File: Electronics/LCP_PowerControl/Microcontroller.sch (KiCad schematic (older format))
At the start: 22 parts, among them J5 Conn_02x05_Odd_Even, J6 Conn_02x06_Odd_Even, J7 Conn_02x02_Odd_Even, J8 Conn_02x02_Odd_Even, SW1 SW_Push, U3 MSP430FR5989, Y1 32.768kHz

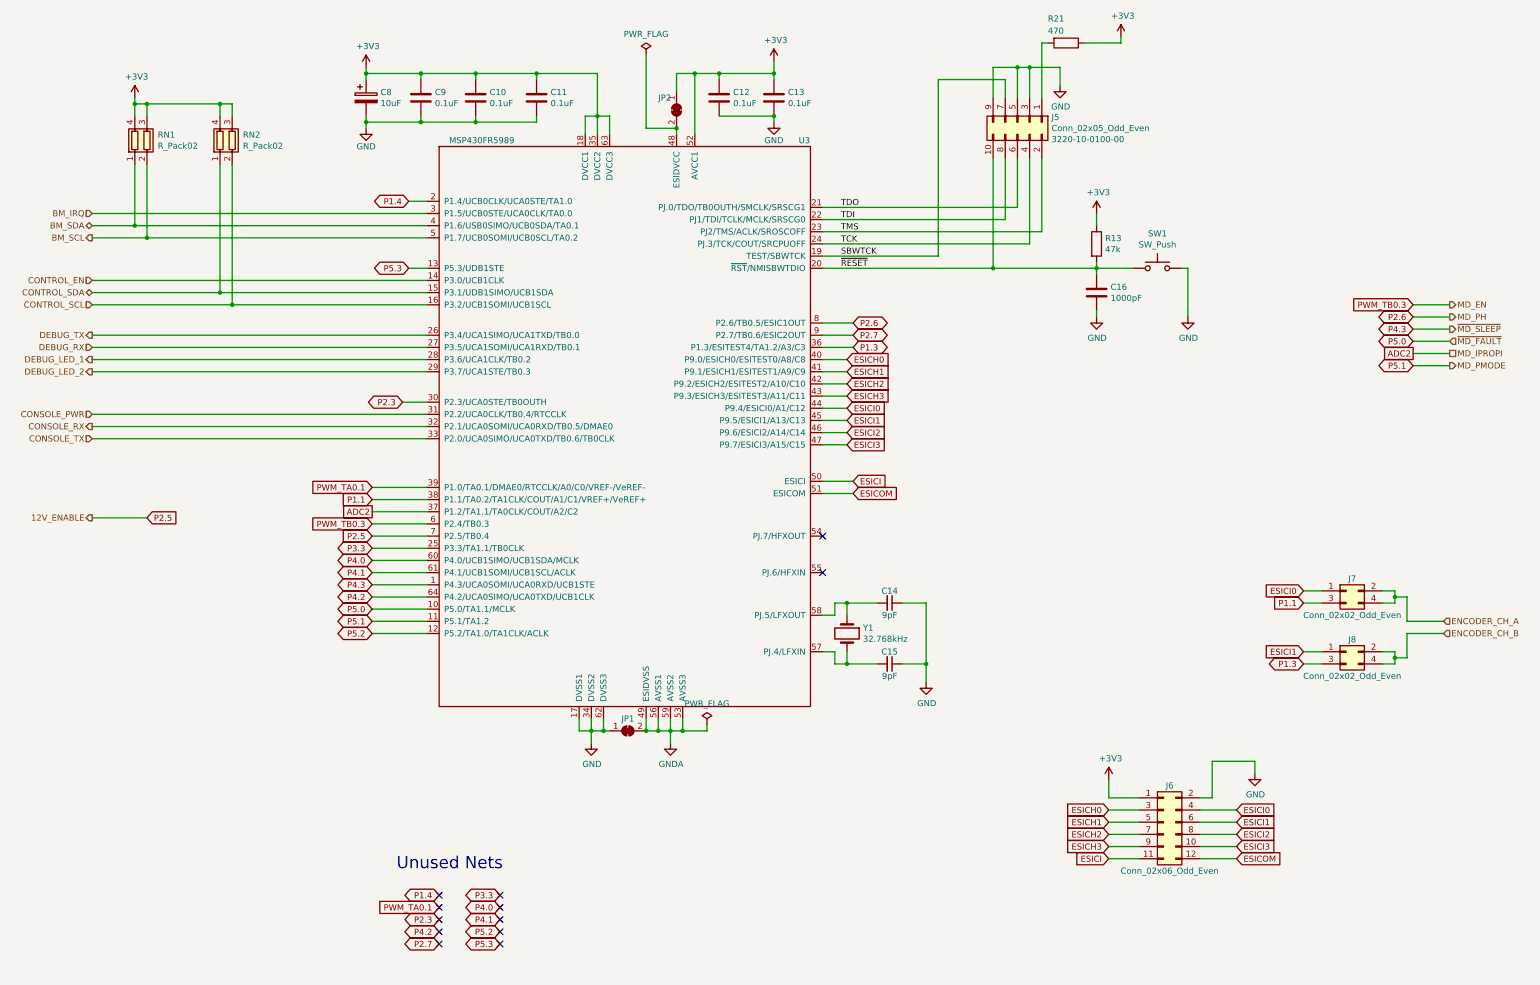
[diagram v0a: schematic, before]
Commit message: Rev 1 Update
Issues #9-#13 fixed
Rev 1 Gerbers & BOM Ready
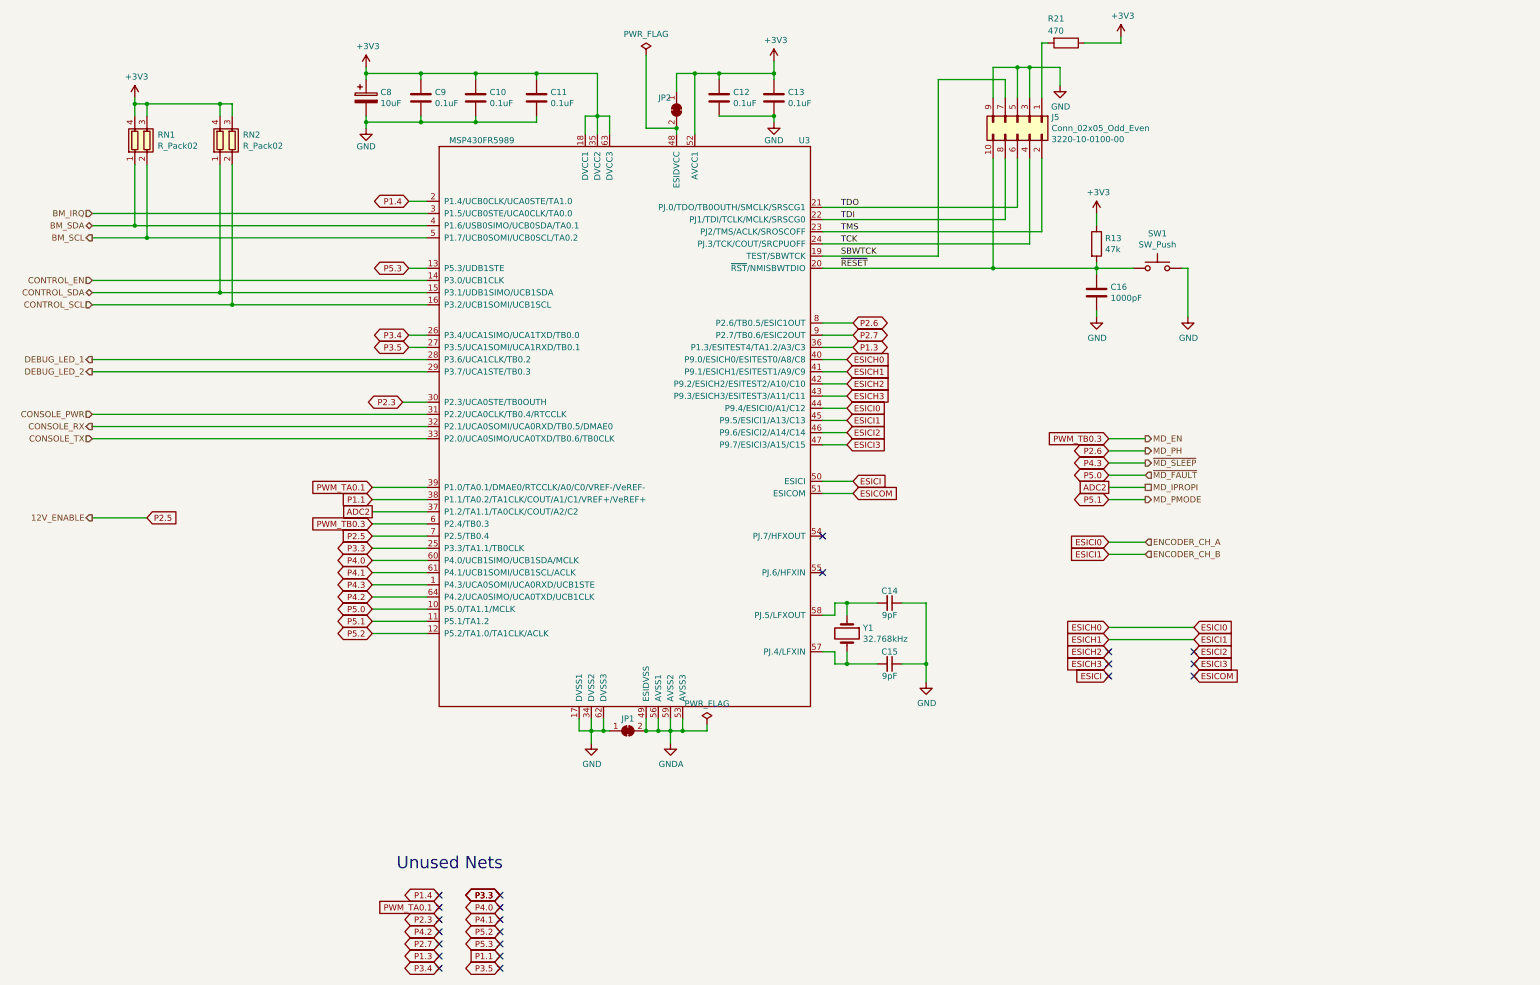
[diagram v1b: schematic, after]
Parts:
- removed J6: Conn_02x06_Odd_Even, Connector_PinHeader_2.00mm:PinHeader_2x06_P2.00mm_Vertical, symbol Connector_Generic:Conn_02x06_Odd_Even
- removed J7, J8: Conn_02x02_Odd_Even, Connector_PinHeader_2.00mm:PinHeader_2x02_P2.00mm_Vertical, symbol Connector_Generic:Conn_02x02_Odd_Even
- C14, C15: MPN CBR06C909B5GAC -> CBR06C909BAGAC
- C16: MPN GCJ188R72A102KA01D -> CL10B102KB8NNNC
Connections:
- net ESICI0 is gone; now on net ESICH0: U3.44 (P9.4/ESICI0/A1/C12)
- net ESICI1 is gone; now on net ESICH1: U3.45 (P9.5/ESICI1/A13/C13)
- net DEBUG_RX renamed P3.5
- net DEBUG_TX renamed P3.4
- no-connect marks 12 -> 22
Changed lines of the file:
@@
 Text HLabel 3900 4800 0    50   Output ~ 0
 CONSOLE_RX
-Text HLabel 15050 3800 2    50   Output ~ 0
+Text HLabel 12550 4900 2    50   Output ~ 0
 MD_EN
-Text HLabel 15050 3900 2    50   Output ~ 0
+Text HLabel 12550 5000 2    50   Output ~ 0
 MD_PH
-Text HLabel 15050 4100 2    50   Input ~ 0
+Text HLabel 12550 5200 2    50   Input ~ 0
 ~MD_FAULT
-Text HLabel 15050 4200 2    50   UnSpc ~ 0
+Text HLabel 12550 5300 2    50   UnSpc ~ 0
 MD_IPROPI
-Text HLabel 15050 4300 2    50   Output ~ 0
+Text HLabel 12550 5400 2    50   Output ~ 0
 MD_PMODE
-Text HLabel 15050 4000 2    50   Output ~ 0
+Text HLabel 12550 5100 2    50   Output ~ 0
 ~MD_SLEEP
 Text HLabel 3900 5550 0    50   Output ~ 0
@@
 F 2 "Capacitor_SMD:C_0603_1608Metric" H 10450 6250 50  0001 C CNN
 F 3 "~" H 10450 6250 50  0001 C CNN
-F 4 "CBR06C909B5GAC" V 10450 6250 50  0001 C CNN "MPN"
+F 4 "CBR06C909BAGAC" V 10450 6250 50  0001 C CNN "MPN"
 	1    10450 6250
 	0    1    1    0
@@
 F 2 "Capacitor_SMD:C_0603_1608Metric" H 10450 6750 50  0001 C CNN
 F 3 "~" H 10450 6750 50  0001 C CNN
-F 4 "CBR06C909B5GAC" V 10450 6750 50  0001 C CNN "MPN"
+F 4 "CBR06C909BAGAC" V 10450 6750 50  0001 C CNN "MPN"
 	1    10450 6750
 	0    1    1    0
@@
 F 2 "Capacitor_SMD:C_0603_1608Metric" H 12188 3550 50  0001 C CNN
 F 3 "~" H 12150 3700 50  0001 C CNN
-F 4 "GCJ188R72A102KA01D" H 12150 3700 50  0001 C CNN "MPN"
+F 4 "CL10B102KB8NNNC" H 12150 3700 50  0001 C CNN "MPN"
 	1    12150 3700
 	1    0    0    -1
@@
 Wire Wire Line
 	6650 5300 6200 5300
-Text HLabel 3900 4050 0    50   Output ~ 0
-DEBUG_TX
-Wire Wire Line
-	3900 4050 6650 4050
-Text HLabel 3900 4150 0    50   Input ~ 0
-DEBUG_RX
-Wire Wire Line
-	3900 4150 6650 4150
 Text HLabel 3900 4250 0    50   Output ~ 0
 DEBUG_LED_1
@@
 P4.2
 Wire Wire Line
-	14750 3900 15050 3900
-Text GLabel 14750 4000 0    50   BiDi ~ 0
+	12250 5000 12550 5000
+Text GLabel 12250 5100 0    50   BiDi ~ 0
 P4.3
 Wire Wire Line
-	14750 4000 15050 4000
-Text GLabel 14750 4100 0    50   BiDi ~ 0
+	12250 5100 12550 5100
+Text GLabel 12250 5200 0    50   BiDi ~ 0
 P5.0
 Wire Wire Line
-	14750 4100 15050 4100
+	12250 5200 12550 5200
 Text GLabel 6200 5500 0    50   UnSpc ~ 0
 ADC2
 Wire Wire Line
 	6200 5500 6650 5500
-Text GLabel 14750 3800 0    50   Input ~ 0
+Text GLabel 12250 4900 0    50   Input ~ 0
 PWM_TB0.3
-Text GLabel 14750 4200 0    50   UnSpc ~ 0
+Text GLabel 12250 5300 0    50   UnSpc ~ 0
 ADC2
 Wire Wire Line
-	14750 4200 15050 4200
-Text GLabel 14750 4300 0    50   BiDi ~ 0
+	12250 5300 12550 5300
+Text GLabel 12250 5400 0    50   BiDi ~ 0
 P5.1
 Wire Wire Line
-	14750 4300 15050 4300
-Text GLabel 12250 7950 0    50   Input ~ 0
+	12250 5400 12550 5400
+Text GLabel 12250 6450 0    50   Input ~ 0
 ESICH0
-Text GLabel 12250 8050 0    50   Input ~ 0
+Text GLabel 12250 6550 0    50   Input ~ 0
 ESICH1
-Text GLabel 12250 8150 0    50   Input ~ 0
+Text GLabel 12250 6650 0    50   Input ~ 0
 ESICH2
-Text GLabel 12250 8250 0    50   Input ~ 0
+Text GLabel 12250 6750 0    50   Input ~ 0
 ESICH3
-Text GLabel 13300 7950 2    50   Input ~ 0
+Text GLabel 12950 6550 2    50   Input ~ 0
+ESICI1
+Text GLabel 12950 6650 2    50   Input ~ 0
+ESICI2
+Text GLabel 12950 6750 2    50   Input ~ 0
+ESICI3
+Text GLabel 12250 6850 0    50   Input ~ 0
+ESICI
+Text GLabel 12950 6850 2    50   Input ~ 0
+ESICOM
+Text HLabel 12550 5750 2    50   Input ~ 0
+ENCODER_CH_A
+Text HLabel 12550 5850 2    50   Input ~ 0
+ENCODER_CH_B
+Text GLabel 12250 5750 0    50   Input ~ 0
 ESICI0
-Text GLabel 13300 8050 2    50   Input ~ 0
+Text GLabel 12250 5850 0    50   Input ~ 0
 ESICI1
-Text GLabel 13300 8150 2    50   Input ~ 0
-ESICI2
-Text GLabel 13300 8250 2    50   Input ~ 0
-ESICI3
-$Comp
-L Connector_Generic:Conn_02x06_Odd_Even J6
-U 1 1 5F0F003E
-P 12700 8050
-F 0 "J6" H 12750 8350 50  0000 C CNN
-F 1 "Conn_02x06_Odd_Even" H 12750 7650 50  0000 C CNN
-F 2 "Connector_PinHeader_2.00mm:PinHeader_2x06_P2.00mm_Vertical" H 12700 8050 50  0001 C CNN
-F 3 "~" H 12700 8050 50  0001 C CNN
-F 4 "2842126-6" H 12700 8050 50  0001 C CNN "MPN"
-	1    12700 8050
-	1    0    0    -1
-$EndComp
-Text GLabel 12250 8350 0    50   Input ~ 0
-ESICI
-Text GLabel 13300 8350 2    50   Input ~ 0
-ESICOM
-Wire Wire Line
-	13300 8350 13000 8350
-Wire Wire Line
-	13000 8250 13300 8250
-Wire Wire Line
-	13300 8150 13000 8150
-Wire Wire Line
-	13000 8050 13300 8050
-Wire Wire Line
-	13300 7950 13000 7950
-Wire Wire Line
-	12500 7950 12250 7950
-Wire Wire Line
-	12250 8050 12500 8050
-Wire Wire Line
-	12500 8150 12250 8150
-Wire Wire Line
-	12250 8250 12500 8250
-Wire Wire Line
-	12250 8350 12500 8350
-$Comp
-L power:GND #PWR031
-U 1 1 5F139610
-P 13450 7650
-F 0 "#PWR031" H 13450 7400 50  0001 C CNN
-F 1 "GND" H 13455 7477 50  0000 C CNN
-F 2 "" H 13450 7650 50  0001 C CNN
-F 3 "" H 13450 7650 50  0001 C CNN
-	1    13450 7650
-	1    0    0    -1
-$EndComp
-Wire Wire Line
-	13000 7850 13100 7850
-Wire Wire Line
-	13100 7850 13100 7550
-Wire Wire Line
-	13100 7550 13450 7550
-Wire Wire Line
-	13450 7550 13450 7650
-$Comp
-L power:+3V3 #PWR030
-U 1 1 5F141006
-P 12250 7700
-F 0 "#PWR030" H 12250 7550 50  0001 C CNN
-F 1 "+3V3" H 12265 7873 50  0000 C CNN
-F 2 "" H 12250 7700 50  0001 C CNN
-F 3 "" H 12250 7700 50  0001 C CNN
-	1    12250 7700
-	1    0    0    -1
-$EndComp
-Wire Wire Line
-	12250 7700 12250 7850
-Wire Wire Line
-	12250 7850 12500 7850
-Text HLabel 15000 6400 2    50   Input ~ 0
-ENCODER_CH_A
-Text HLabel 15000 6500 2    50   Input ~ 0
-ENCODER_CH_B
-Text GLabel 13850 6150 0    50   Input ~ 0
-ESICI0
-Text GLabel 13850 6650 0    50   Input ~ 0
-ESICI1
-$Comp
-L Connector_Generic:Conn_02x02_Odd_Even J7
-U 1 1 5F17BAA5
-P 14200 6150
-F 0 "J7" H 14250 6250 50  0000 C CNN
-F 1 "Conn_02x02_Odd_Even" H 14250 5950 50  0000 C CNN
-F 2 "Connector_PinHeader_2.00mm:PinHeader_2x02_P2.00mm_Vertical" H 14200 6150 50  0001 C CNN
-F 3 "~" H 14200 6150 50  0001 C CNN
-F 4 "5176264-1" H 14200 6150 50  0001 C CNN "MPN"
-	1    14200 6150
-	1    0    0    -1
-$EndComp
-$Comp
-L Connector_Generic:Conn_02x02_Odd_Even J8
-U 1 1 5F17C61B
-P 14200 6650
-F 0 "J8" H 14250 6750 50  0000 C CNN
-F 1 "Conn_02x02_Odd_Even" H 14250 6450 50  0000 C CNN
-F 2 "Connector_PinHeader_2.00mm:PinHeader_2x02_P2.00mm_Vertical" H 14200 6650 50  0001 C CNN
-F 3 "~" H 14200 6650 50  0001 C CNN
-F 4 "5176264-1" H 14200 6650 50  0001 C CNN "MPN"
-	1    14200 6650
-	1    0    0    -1
-$EndComp
-Wire Wire Line
-	14500 6150 14600 6150
-Wire Wire Line
-	14600 6150 14600 6200
-Wire Wire Line
-	14600 6250 14500 6250
-Wire Wire Line
-	14500 6650 14600 6650
-Wire Wire Line
-	14600 6650 14600 6700
-Wire Wire Line
-	14600 6750 14500 6750
-Wire Wire Line
-	14600 6700 14700 6700
-Wire Wire Line
-	14700 6700 14700 6500
-Wire Wire Line
-	14700 6500 15000 6500
-Connection ~ 14600 6700
-Wire Wire Line
-	14600 6700 14600 6750
-Wire Wire Line
-	15000 6400 14700 6400
-Wire Wire Line
-	14700 6400 14700 6200
-Wire Wire Line
-	14700 6200 14600 6200
-Connection ~ 14600 6200
-Wire Wire Line
-	14600 6200 14600 6250
-Wire Wire Line
-	14000 6650 13850 6650
-Wire Wire Line
-	14000 6150 13850 6150
-Text GLabel 13850 6250 0    50   Input ~ 0
-P1.1
-Wire Wire Line
-	13850 6250 14000 6250
+Wire Wire Line
+	12250 5850 12550 5850
+Wire Wire Line
+	12550 5750 12250 5750
 Text GLabel 4350 5550 2    50   Input ~ 0
 P2.5
@@
 Wire Wire Line
 	10150 3950 9900 3950
-Text GLabel 14750 3900 0    50   BiDi ~ 0
+Text GLabel 12250 5000 0    50   BiDi ~ 0
 P2.6
 Text GLabel 6750 9050 0    50   BiDi ~ 0
 P2.7
-Text GLabel 13850 6750 0    50   BiDi ~ 0
+Text GLabel 6750 9150 0    50   BiDi ~ 0
 P1.3
 Text GLabel 6450 4600 0    50   BiDi ~ 0
@@
 Connection ~ 4250 3150
 Wire Wire Line
-	13850 6750 14000 6750
-Wire Wire Line
-	14750 3800 15050 3800
+	12250 4900 12550 4900
 Text HLabel 3900 4700 0    50   Input ~ 0
 CONSOLE_PWR
@@
 	0    1    1    0
 $EndComp
+Text GLabel 7250 8650 0    50   BiDi ~ 0
+P3.3
+Text GLabel 7250 9150 0    50   Input ~ 0
+P1.1
+NoConn ~ 6750 9150
+NoConn ~ 7250 9150
+Text GLabel 12950 6450 2    50   Input ~ 0
+ESICI0
+Wire Wire Line
+	12250 6450 12950 6450
+Wire Wire Line
+	12950 6550 12250 6550
+Text GLabel 6750 9250 0    50   BiDi ~ 0
+P3.4
+Text GLabel 7250 9250 0    50   BiDi ~ 0
+P3.5
+NoConn ~ 6750 9250
+NoConn ~ 7250 9250
+NoConn ~ 12250 6650
+NoConn ~ 12250 6750
+NoConn ~ 12250 6850
+NoConn ~ 12950 6850
+NoConn ~ 12950 6750
+NoConn ~ 12950 6650
+Text GLabel 6500 4050 0    50   BiDi ~ 0
+P3.4
+Wire Wire Line
+	6500 4050 6650 4050
+Text GLabel 6500 4150 0    50   BiDi ~ 0
+P3.5
+Wire Wire Line
+	6650 4150 6500 4150
 $EndSCHEMATC
